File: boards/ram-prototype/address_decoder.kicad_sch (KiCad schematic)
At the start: 33 parts, among them U1 74LVC1G04, U10 74LVC1G11, U11 74LVC1G11, U2 74LVC1G04, U3 74LVC1G04, U4 74LVC1G11, U5 74LVC1G11, U6 74LVC1G11, U7 74LVC1G11, U8 74LVC1G11, U9 74LVC1G11

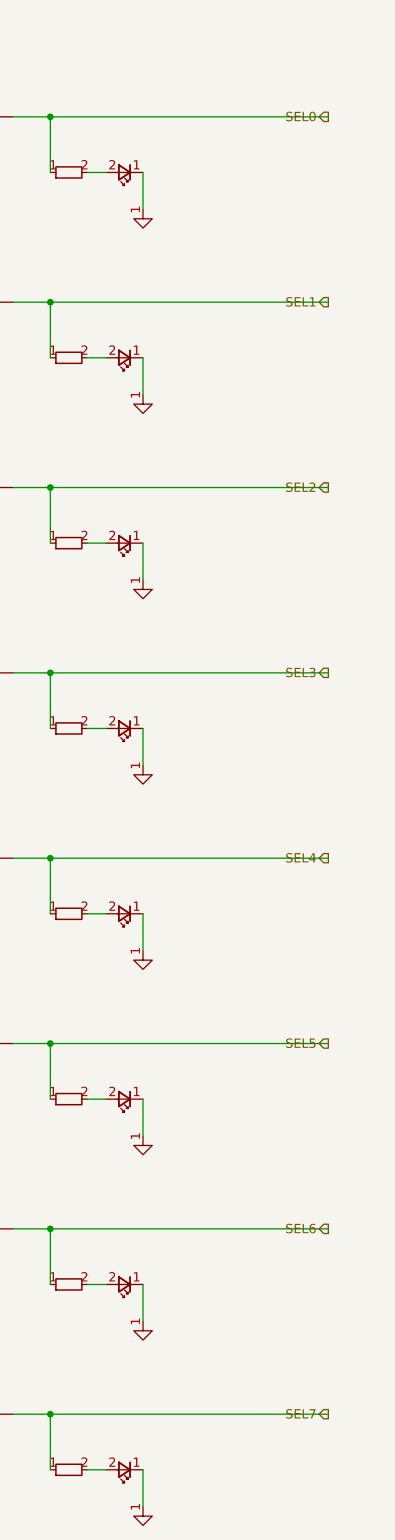
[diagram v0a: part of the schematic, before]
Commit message: Clean up root more and add more data
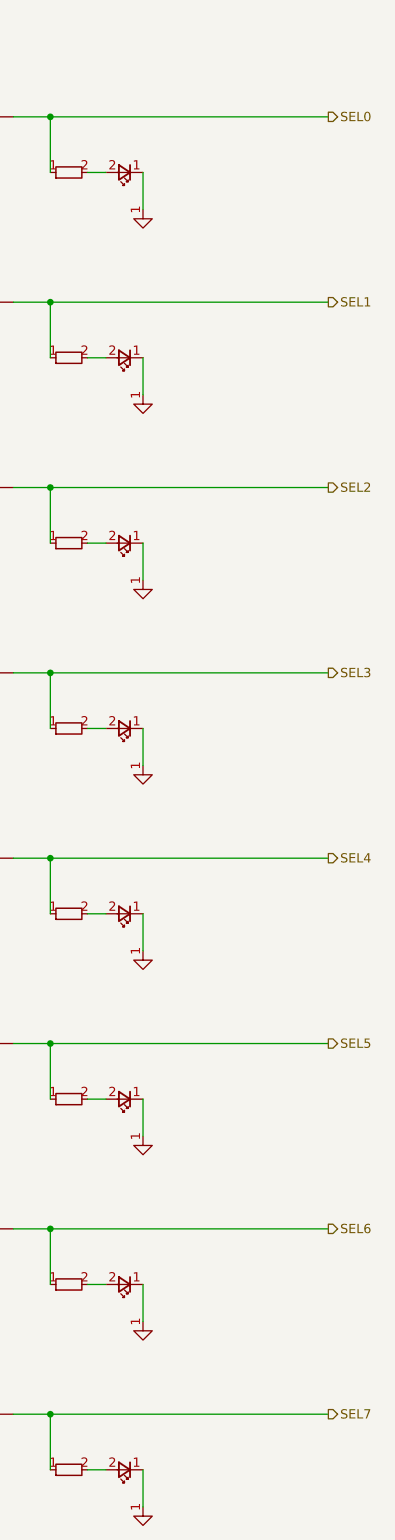
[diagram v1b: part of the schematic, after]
